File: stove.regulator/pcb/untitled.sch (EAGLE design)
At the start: 6 parts, among them IC1 4051N

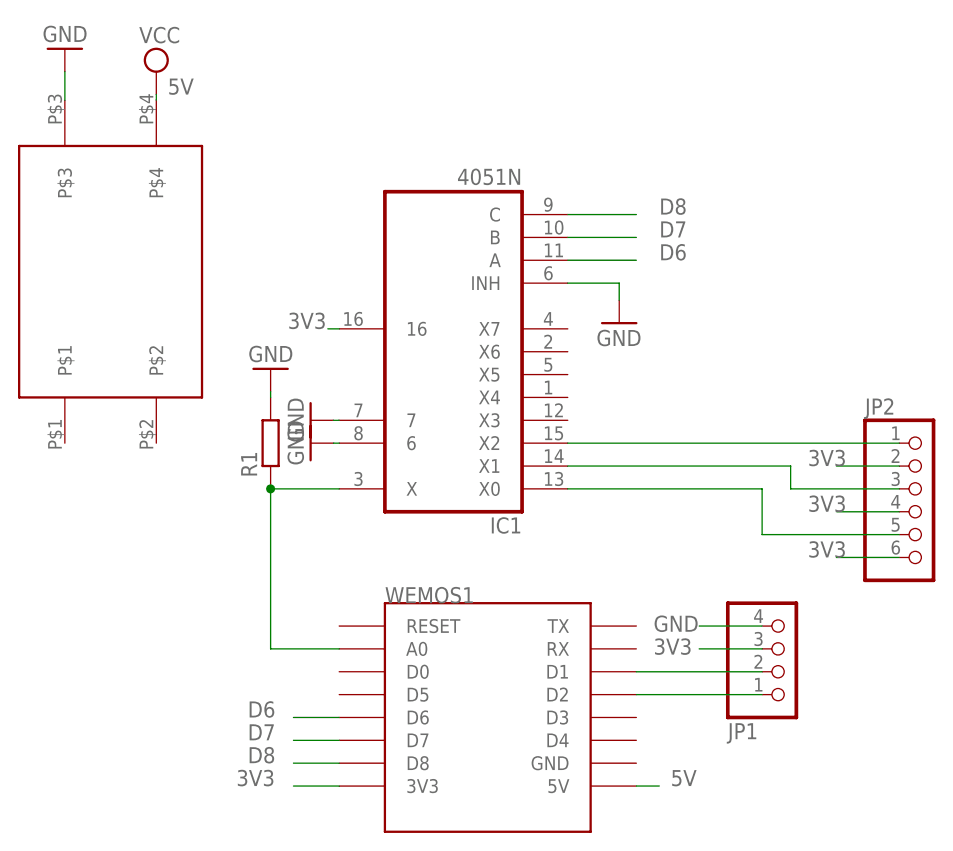
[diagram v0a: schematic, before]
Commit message: part of config
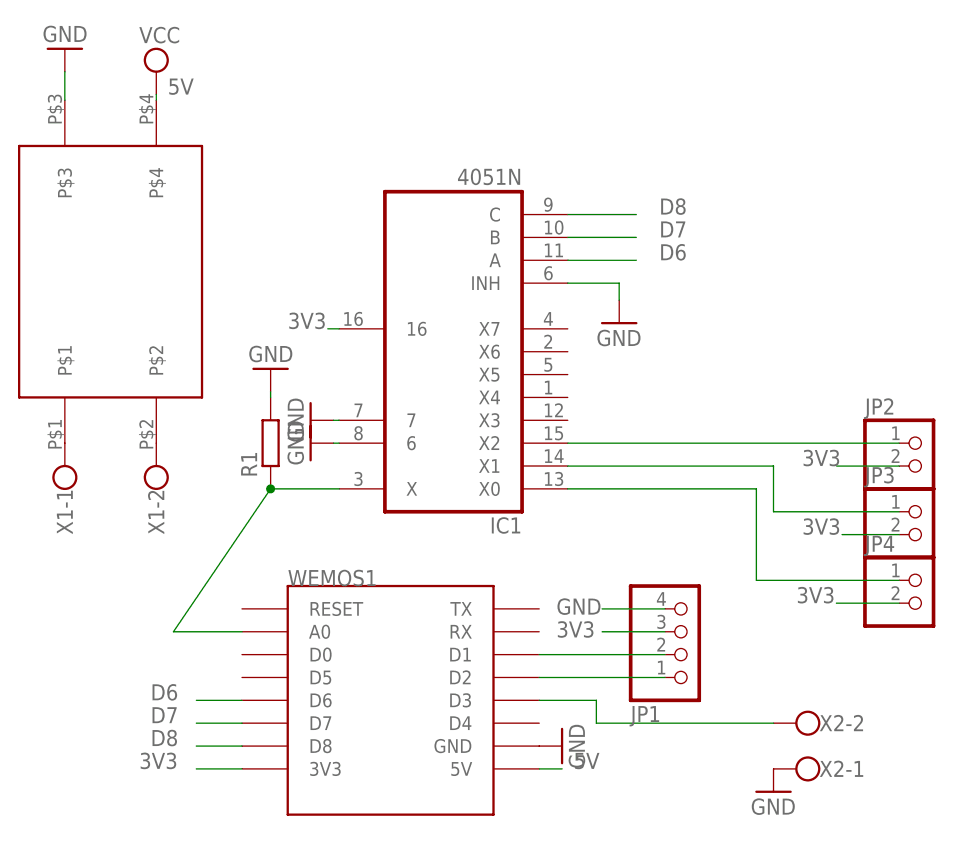
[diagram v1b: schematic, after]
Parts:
- added JP3, JP4: (no value), pinhead:PINHD-1X2
- added X1, X2: (no value), con-wago-500:W237-102
- JP2: device pinhead:PINHD-1X6 -> pinhead:PINHD-1X2
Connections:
- new net N$7: U$6.P$1, X1-1.KL
- new net N$8: U$6.P$2, X1-2.KL
- new net N$9: WEMOS1.D3, X2-2.KL
- net 3V3: now also JP3.2, JP4.2; no longer JP2.4, JP2.6
- net GND: now also WEMOS1.GND, X2-1.KL
- net N$2: now also JP4.1; no longer JP2.5
- net N$3: now also JP3.1; no longer JP2.3
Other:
- moved on the sheet: JP1, WEMOS1
